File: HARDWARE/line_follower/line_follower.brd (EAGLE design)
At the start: 85.4 x 88.9 mm, 74 parts, among them IC1 L3GD20HSMD, IC2 L6205, IC3 ATMEGA328PMA, IC4 LF33, J1 FFC2B05-10-X_REVC, J2 FFC2B05-10-X_REVC, Q1 10MHz, T1 ELPT15-21C, T2 ELPT15-21C, T3 ELPT15-21C, T4 ELPT15-21C, T5 ELPT15-21C, T6 ELPT15-21C, X1 MINI-USB-SCHIELD-32005-301

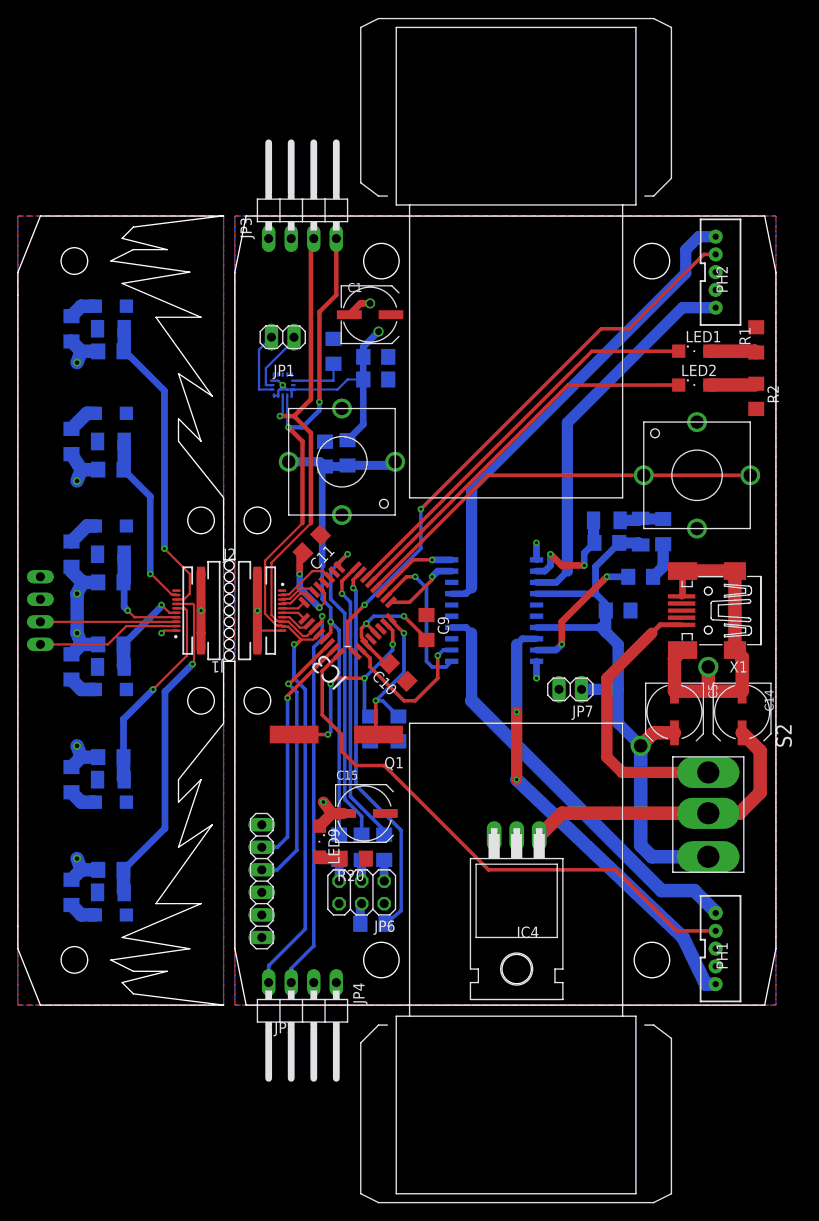
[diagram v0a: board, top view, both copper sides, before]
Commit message: common
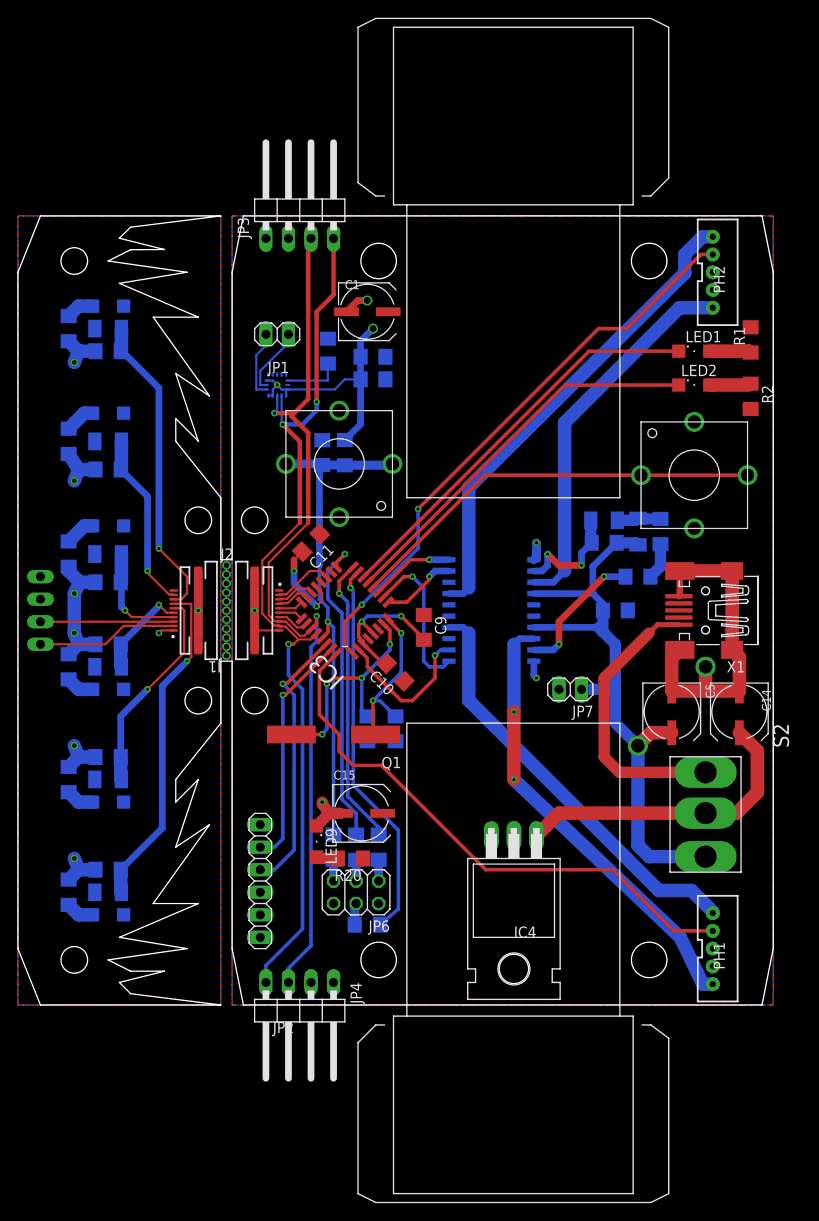
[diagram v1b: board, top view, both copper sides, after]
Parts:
- moved JP1 0.71 mm to (29.2, 75.6)
- moved R1 0.64 mm to (82.5, 74.9)
- moved R2 0.64 mm to (82.5, 68.6)
- moved R19 0.63 mm to (39.4, 9.05)
- moved C4 0.63 mm to (34.9, 73.7)
- moved R16 0.63 mm to (35.6, 17.8)
- moved R17 0.63 mm to (38.1, 17.8)
- moved R18 0.63 mm to (40.6, 17.8)
- moved IC1 0.63 mm to (29.2, 69.8)
- moved JP6 0.63 mm to (38.1, 12.7)
- moved C1 0.45 mm to (39.4, 78.1)
- moved S3 0.39 mm to (36.2, 61.0)
- moved C16 0.35 mm to (34.3, 62.2)
- moved PH2 0.33 mm to (78.1, 82.5)
- moved PH1 0.33 mm to (78.1, 6.35)
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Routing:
- net SCL: track 100.4 -> 101.2 mm
- net N$5: track 5.30 -> 4.66 mm
- net N$13: track 5.30 -> 4.66 mm
- net GND: track 83.8 -> 84.4 mm
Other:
- board size 85.4 x 88.9 mm -> 85.1 x 88.9 mm
- board text removed: "/home/arch/Documents/proj/slate_vixen/HARDWARE/line_follower/printing/dragon_head.bmp"
